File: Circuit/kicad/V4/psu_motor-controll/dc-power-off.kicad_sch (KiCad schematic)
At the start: 12 parts

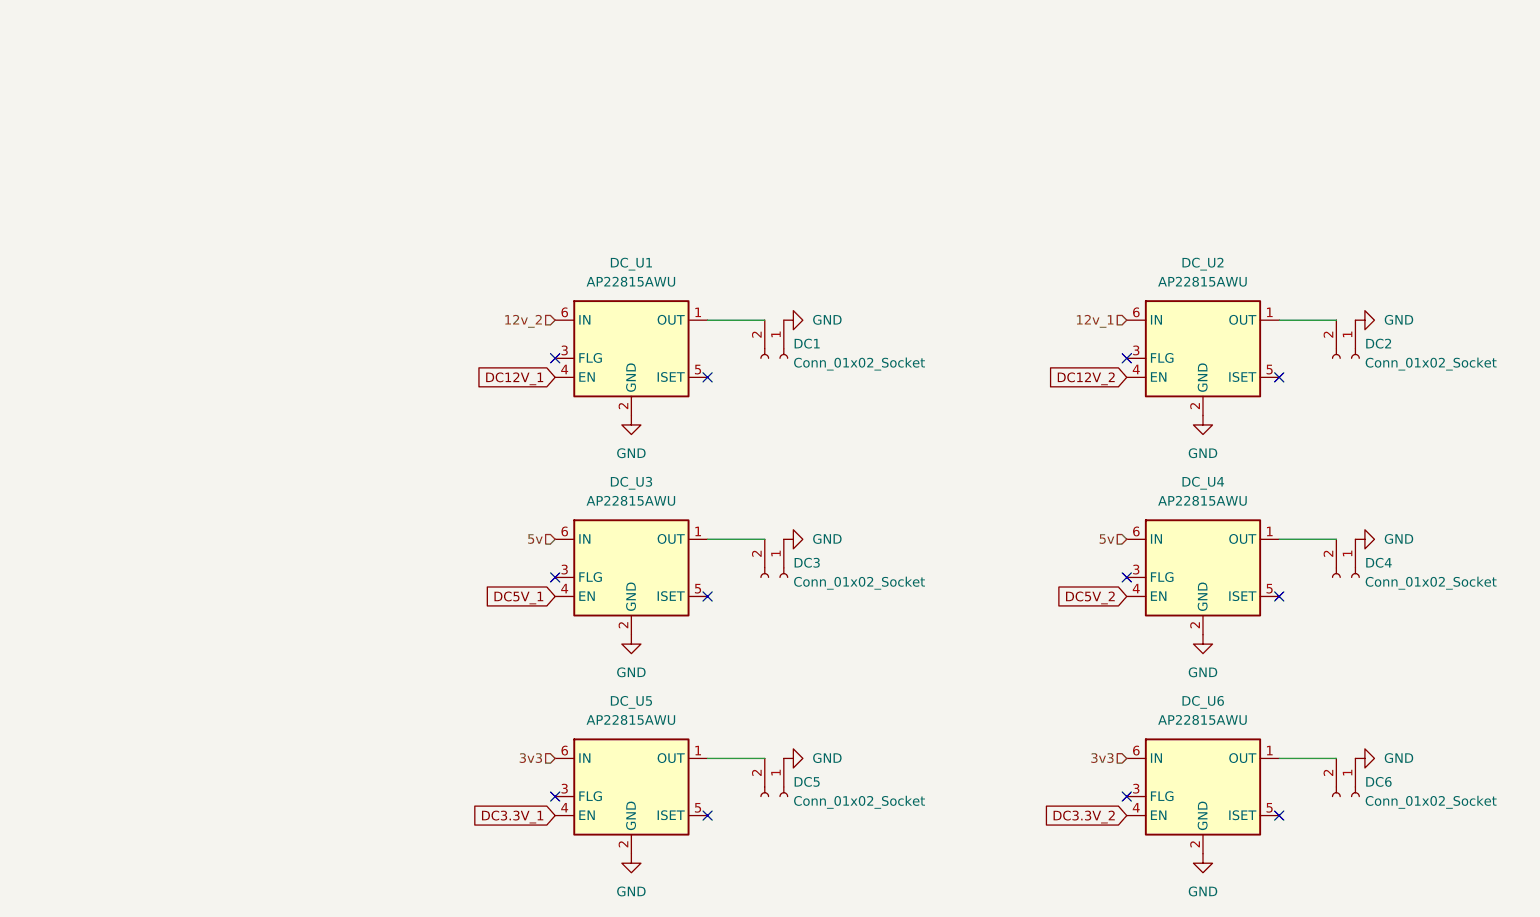
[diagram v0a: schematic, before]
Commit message: PSU FINISH BOARD NO DRC,ERC,DFM ERRORS
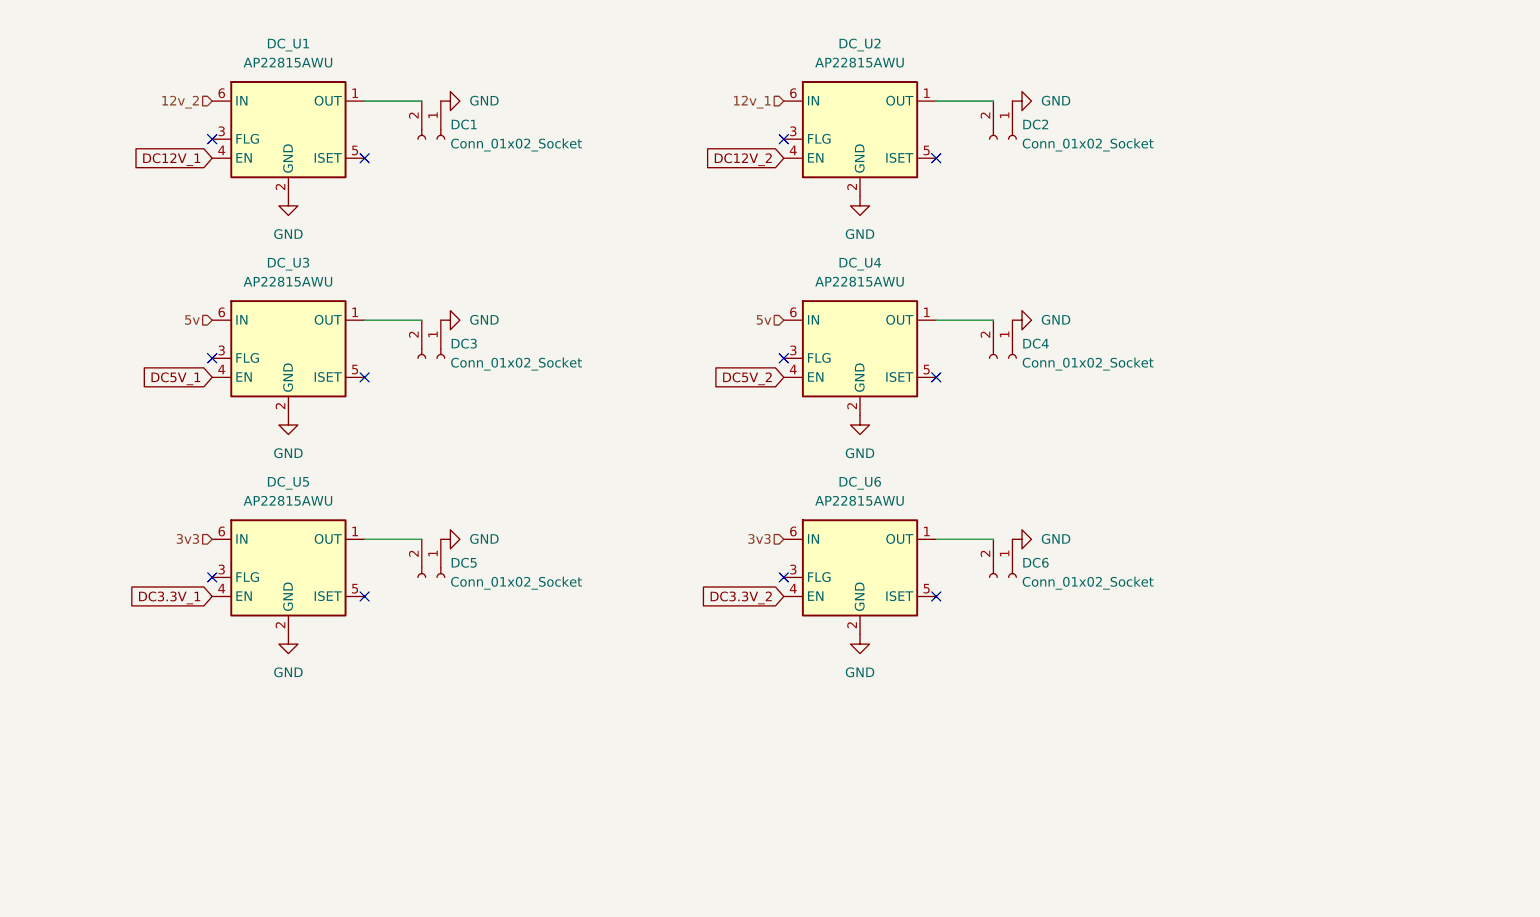
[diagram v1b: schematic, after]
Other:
- moved on the sheet: DC1, DC2, DC3, DC4, DC5, DC6, DC_U1, DC_U2, DC_U3, DC_U4, DC_U5, DC_U6

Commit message: V4.1.7 PSU  V1.0 debug Card
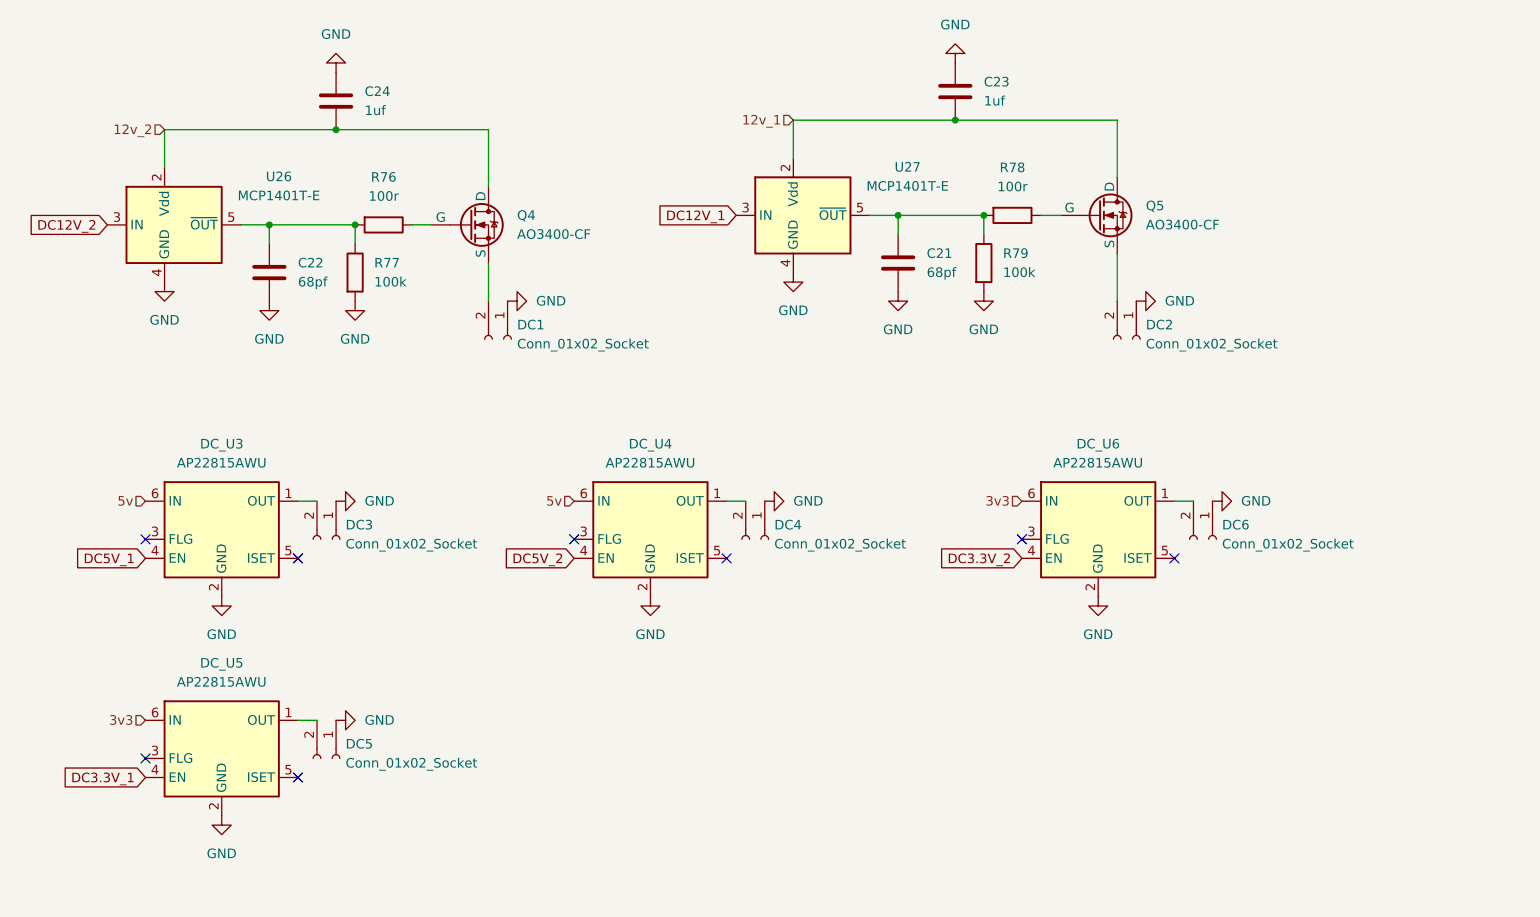
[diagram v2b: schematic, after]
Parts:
- removed DC_U1, DC_U2: AP22815AWU, Package_TO_SOT_SMD:SOT-23-6, symbol Regulator_Linear:AP22615AWU
- added C21, C22: 68pf, Capacitor_SMD:C_0805_2012Metric, symbol Device:C
- added C23, C24: 1uf, Capacitor_SMD:C_0805_2012Metric, symbol Device:C
- added Q4, Q5: AO3400-CF, Package_TO_SOT_SMD:TSOT-23, symbol Simulation_SPICE:NMOS
- added R76, R78: 100r, Resistor_SMD:R_0805_2012Metric, symbol Device:R
- added R77, R79: 100k, Resistor_SMD:R_0805_2012Metric, symbol Device:R
- added U26, U27: MCP1401T-E, Package_TO_SOT_SMD:SOT-23-5, symbol Driver_FET:MCP1415
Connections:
- net 12v_1: now also C23.1, Q5.1 (D), U27.2 (Vdd)
- net 12v_2: now also C24.1, Q4.1 (D), U26.2 (Vdd)
- net DC12V_1: now also U27.3 (IN)
- net DC12V_2: now also U26.3 (IN)
- net GND: now also C21.2, C22.2, C23.2, C24.2, R77.2, R79.2, U26.4 (GND), U27.4 (GND)
- net at DC2.2 (Pin_2): now also Q5.3 (S)
- net at DC1.2 (Pin_2): now also Q4.3 (S)
- new net: C21.1, R78.2, R79.1, U27.5 (~{OUT})
- new net: C22.1, R76.2, R77.1, U26.5 (~{OUT})
- new net: Q5.2 (G), R78.1
- new net: Q4.2 (G), R76.1
- no-connect marks 12 -> 8
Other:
- moved on the sheet: DC1, DC2, DC3, DC4, DC5, DC6, DC_U3, DC_U4, DC_U5, DC_U6
